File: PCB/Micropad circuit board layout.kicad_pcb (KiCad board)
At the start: 2 copper layers, 96 x 56 mm, 47 parts, among them SW1 SW_Push_45deg, SW10 SW_Push_45deg, SW11 SW_Push_45deg, SW12 SW_Push_45deg, SW13 SW_Push_45deg, SW14 SW_Push_45deg, SW15 SW_Push_45deg, SW2 SW_Push_45deg, SW3 SW_Push_45deg, SW4 SW_Push_45deg, SW5 SW_Push_45deg, SW6 SW_Push_45deg, SW7 SW_Push_45deg, SW8 SW_Push_45deg, SW9 SW_Push_45deg, U1 MOUDLE-SEEEDUINO-XIAO

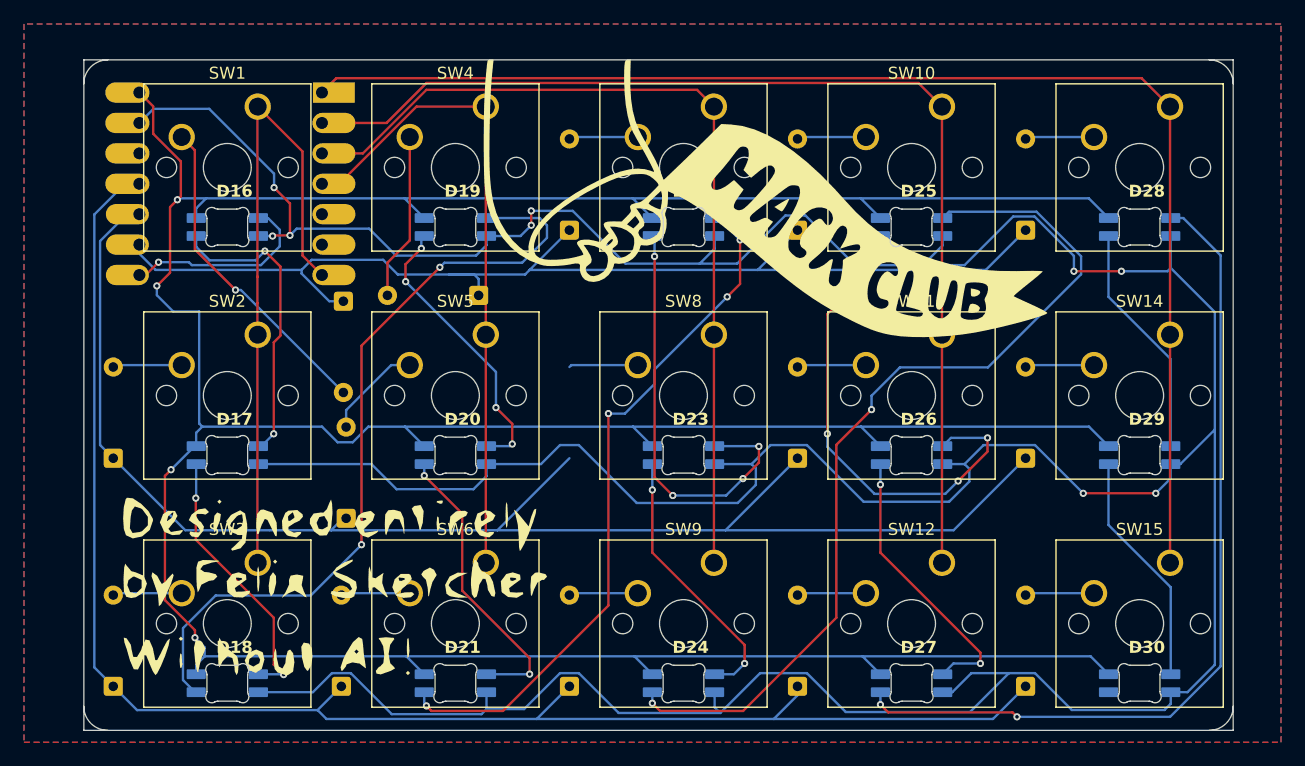
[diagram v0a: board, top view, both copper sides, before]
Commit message: Fixing files
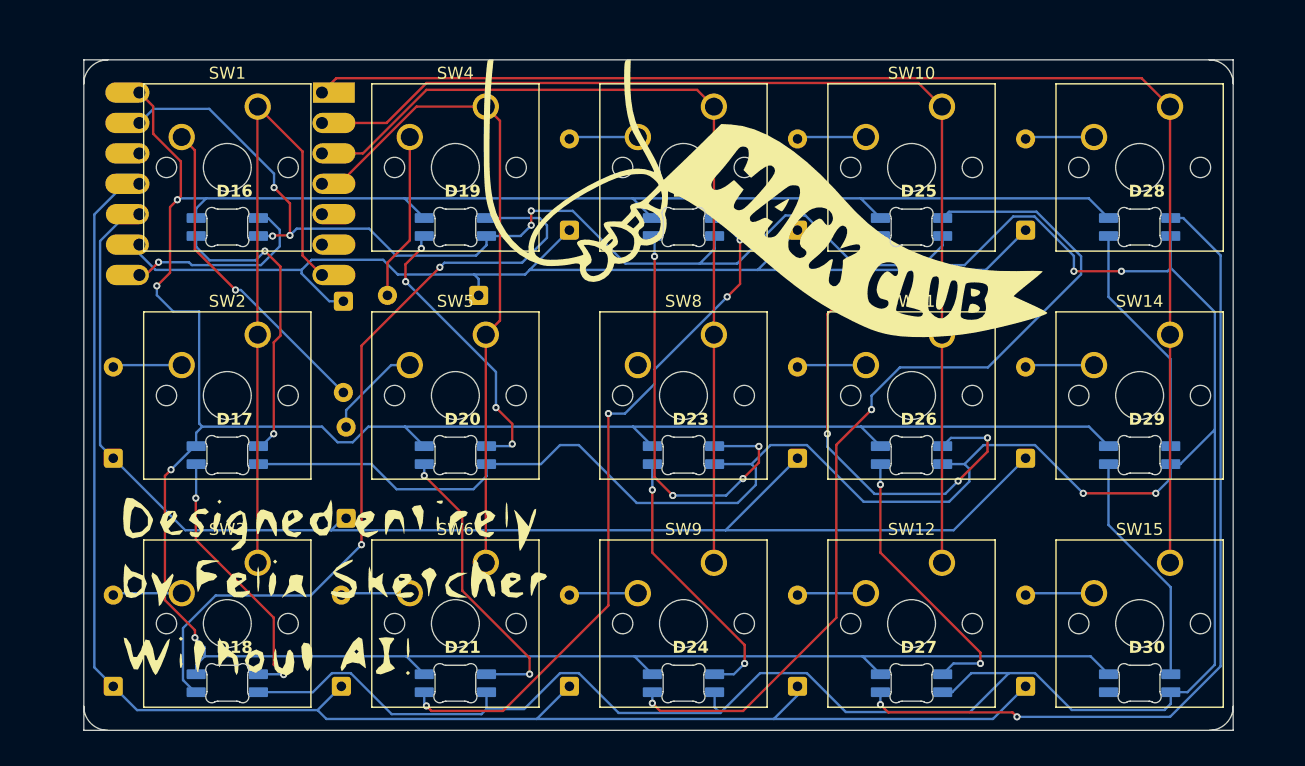
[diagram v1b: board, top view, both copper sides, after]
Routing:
- net /Row_1: track 123.5 -> 114.1 mm
- net Net-(D8-A): track 5.78 -> 0.00 mm
- net /Row_0: track 95.9 -> 93.8 mm
- net /Col_1: track 54.5 -> 55.4 mm
- removed copper zone on B.Cu, net (none)
- removed copper zone on F.Cu, net (none)
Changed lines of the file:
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@@
 			(disableapertmacros no)
 			(usegerberextensions yes)
-			(usegerberattributes yes)
-			(usegerberadvancedattributes yes)
-			(creategerberjobfile yes)
+			(usegerberattributes no)
+			(usegerberadvancedattributes no)
+			(creategerberjobfile no)
 			(dashed_line_dash_ratio 12.000000)
 			(dashed_line_gap_ratio 3.000000)
@@
 			(sketchdnponfab yes)
 			(crossoutdnponfab yes)
-			(subtractmaskfromsilk no)
+			(subtractmaskfromsilk yes)
 			(outputformat 1)
 			(mirror no)
 			(drillshape 0)
 			(scaleselection 1)
-			(outputdirectory "../../")
+			(outputdirectory "../Gerbers/")
 		)
 	)
@@
 	)
 	(segment
-		(start 160.075 80.439)
-		(end 157.975 80.439)
-		(width 0.2)
-		(layer "B.Cu")
-		(net 2)
-	)
-	(segment
 		(start 164.33475 80.439)
 		(end 164.71375 80.06)
@@
 	)
 	(segment
-		(start 142.285 80.06)
-		(end 133.47 80.06)
+		(start 133.47 80.06)
+		(end 145.66375 80.06)
 		(width 0.2)
 		(layer "B.Cu")
@@
 	(segment
 		(start 153.699 80.439)
-		(end 158.401 80.439)
+		(end 164.33475 80.439)
 		(width 0.2)
 		(layer "B.Cu")
@@
 	)
 	(segment
-		(start 158.401 80.439)
-		(end 164.33475 80.439)
-		(width 0.2)
-		(layer "B.Cu")
-		(net 2)
-	)
-	(segment
 		(start 132.115 78.705)
 		(end 132.115 77.945)
@@
 	)
 	(segment
-		(start 142.285 80.06)
-		(end 145.66375 80.06)
-		(width 0.2)
-		(layer "B.Cu")
-		(net 2)
-	)
-	(segment
 		(start 164.71375 80.06)
 		(end 183.76375 80.06)
@@
 	)
 	(segment
-		(start 135.94625 101.8)
-		(end 142.97375 101.8)
-		(width 0.2)
-		(layer "B.Cu")
-		(net 3)
-	)
-	(segment
 		(start 129.935 95.78875)
 		(end 135.94625 101.8)
@@
 	)
 	(segment
-		(start 162.02375 101.8)
-		(end 168.035 95.78875)
-		(width 0.2)
-		(layer "B.Cu")
-		(net 3)
-	)
-	(segment
 		(start 149.13 100.805)
 		(end 148.135 101.8)
@@
 	)
 	(segment
-		(start 148.985 100.135)
-		(end 148.985 100.95)
-		(width 0.2)
-		(layer "B.Cu")
-		(net 3)
-	)
-	(segment
-		(start 142.97375 101.8)
+		(start 135.94625 101.8)
 		(end 148.135 101.8)
 		(width 0.2)
@@
 	)
 	(segment
-		(start 162.02375 101.8)
-		(end 181.07375 101.8)
-		(width 0.2)
-		(layer "B.Cu")
-		(net 3)
-	)
-	(segment
 		(start 131.07724 75.405)
 		(end 128.834 77.64824)
@@
 	(segment
 		(start 148.135 101.8)
-		(end 162.02375 101.8)
+		(end 181.07375 101.8)
 		(width 0.2)
 		(layer "B.Cu")
@@
 	)
 	(segment
-		(start 141.975 82.836)
+		(start 141.975 66.445)
 		(end 141.975 104.495)
 		(width 0.2)
@@
 	)
 	(segment
-		(start 141.96984 82.836)
-		(end 141.975 82.836)
-		(width 0.2)
-		(layer "F.Cu")
-		(net 21)
-	)
-	(segment
-		(start 141.975 66.445)
-		(end 141.975 80.634)
-		(width 0.2)
-		(layer "F.Cu")
-		(net 21)
-	)
-	(segment
-		(start 141.975 80.634)
-		(end 141.96984 80.634)
-		(width 0.2)
-		(layer "F.Cu")
-		(net 21)
-	)
-	(segment
 		(start 142 66.42)
 		(end 141.975 66.445)
@@
 	)
 	(segment
-		(start 141.975 82.836)
-		(end 141.975 80.634)
-		(width 0.2)
-		(layer "F.Cu")
-		(net 21)
-	)
-	(segment
 		(start 145.741 78.861)
 		(end 147.365 80.485)
@@
 	)
 	(segment
+		(start 155.258686 66.42)
+		(end 148.813686 72.865)
+		(width 0.2)
+		(layer "F.Cu")
+		(net 22)
+	)
+	(segment
+		(start 162.235 67.605)
+		(end 162.235 84.285)
+		(width 0.2)
+		(layer "F.Cu")
+		(net 22)
+	)
+	(segment
 		(start 161.05 66.42)
-		(end 161.05 85.47)
+		(end 162.235 67.605)
 		(width 0.2)
 		(layer "F.Cu")
@@
 	)
 	(segment
-		(start 155.258686 66.42)
-		(end 148.813686 72.865)
+		(start 162.235 84.285)
+		(end 161.05 85.47)
 		(width 0.2)
 		(layer "F.Cu")
@@
 	)
 	(segment
-		(start 197.3721 64.075)
-		(end 197.3411 64.044)
-		(width 0.2)
-		(layer "F.Cu")
-		(net 25)
-	)
-	(segment
 		(start 218.2 66.42)
 		(end 215.824 64.044)
@@
 	)
 	(segment
-		(start 133.605 79.305)
-		(end 133.715 79.415)
-		(width 0.2)
-		(layer "F.Cu")
-		(net 26)
-	)
-	(segment
 		(start 132.115 80.485)
 		(end 132.645 80.485)
@@
 	)
 	(segment
-		(start 175.145 78.93)
-		(end 175.145 78.92)
-		(width 0.2)
-		(layer "B.Cu")
-		(net 33)
-	)
-	(segment
 		(start 181.12 98.9)
 		(end 182.53 97.49)
@@
 	)
 	(segment
-		(start 168.19375 88.01)
-		(end 168.035 88.16875)
-		(width 0.2)
-		(layer "B.Cu")
-		(net 43)
-	)
-	(segment
-		(start 173.75 88.01)
-		(end 168.19375 88.01)
-		(width 0.2)
-		(layer "B.Cu")
-		(net 43)
-	)
-	(segment
 		(start 173.75 107.06)
 		(end 168.19375 107.06)
@@
 		(net 44)
 	)
-	(zone
-		(net 0)
-		(net_name "")
-		(layers "F.Cu" "B.Cu")
-		(hatch edge 0.5)
-		(connect_pads
-			(clearance 0.5)
-		)
-		(min_thickness 0.25)
-		(filled_areas_thickness no)
-		(fill yes
-			(thermal_gap 0.5)
-			(thermal_bridge_width 0.5)
-			(island_removal_mode 1)
-			(island_area_min 10)
-		)
-		(polygon
-			(pts
-				(xy 227.475 59.515) (xy 122.475 59.515) (xy 122.475 119.515) (xy 227.475 119.515)
-			)
-		)
-	)
 	(embedded_fonts no)
